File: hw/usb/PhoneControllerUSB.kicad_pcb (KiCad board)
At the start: 2 copper layers, 28.1 x 17 mm, 4 parts, among them J1 525590652, J2 DX07VN24WA2C1568

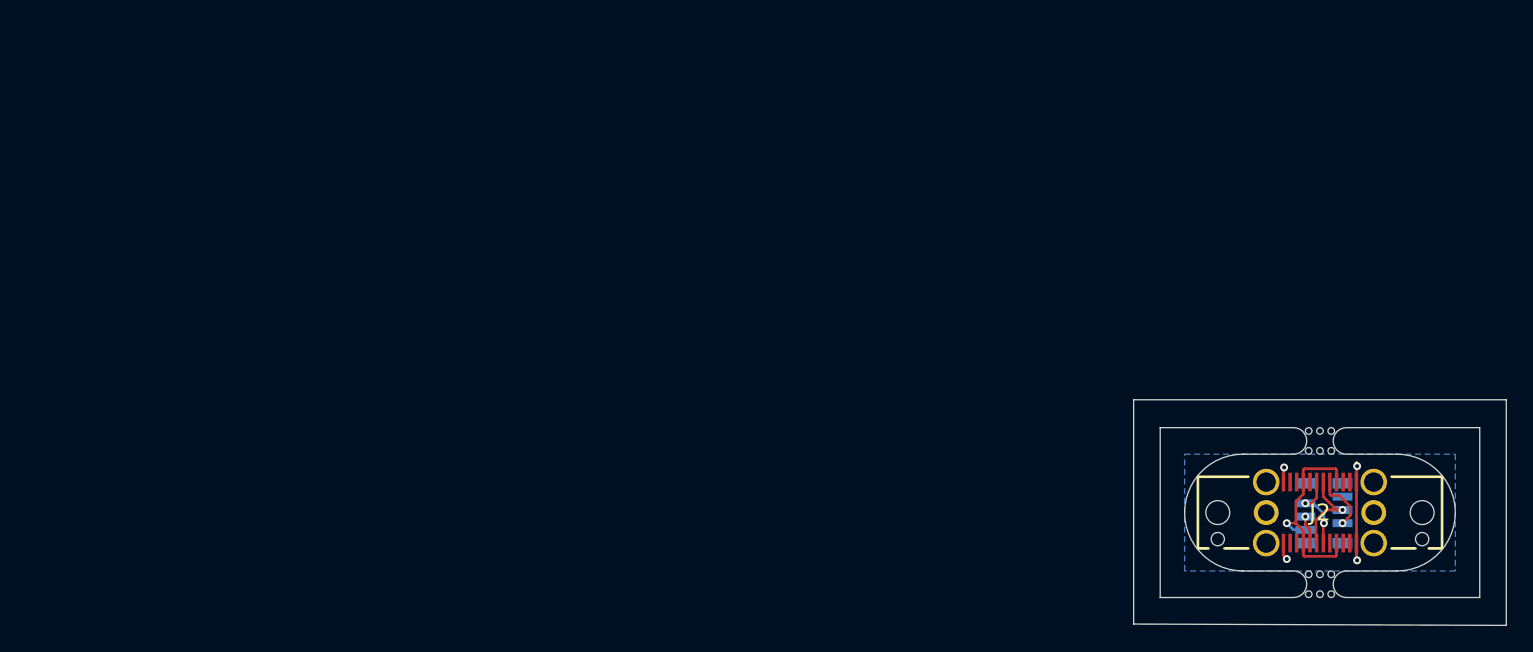
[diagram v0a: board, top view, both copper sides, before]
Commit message: chore: Updating schematics
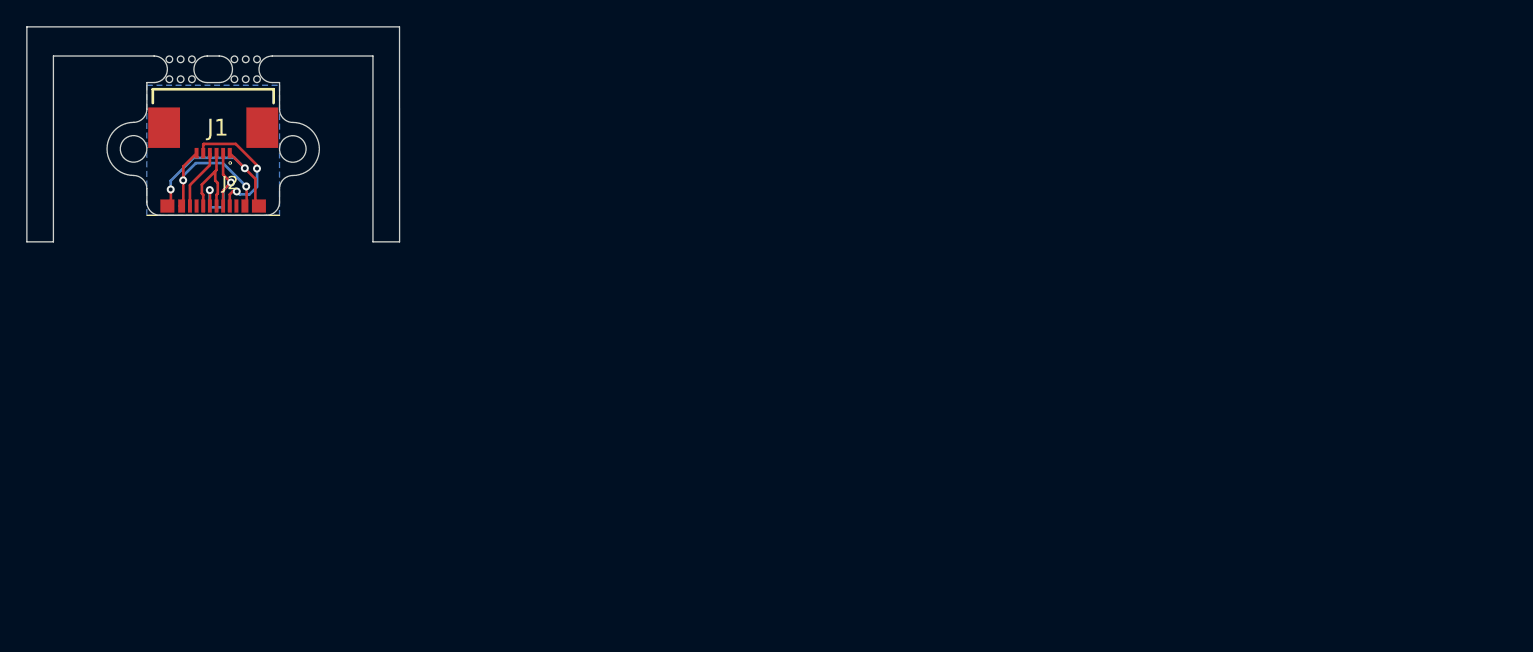
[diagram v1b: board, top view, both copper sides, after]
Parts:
- removed the REF** at (83.4, 34.0)
- removed the REF** at (83.4, 23.2)
- added REF**: MouseBite-Slot_2.0x2.0mm_outset_D0.5mm_P0.85mm_3h, Panelization:MouseBite-Slot_2.0x2.0mm_outset_D0.5mm_P0.85mm_3h, F.Cu at (2.45, -4.80)
- added REF**: MouseBite-Slot_2.0x2.0mm_outset_D0.5mm_P0.85mm_3h, Panelization:MouseBite-Slot_2.0x2.0mm_outset_D0.5mm_P0.85mm_3h, F.Cu at (-2.45, -4.80)
- J1: footprint 52559-0652:CON_525590652_MOL -> 52746-0671:52746-0671; moved to F.Cu
- J2: footprint DX07VN24WA2C1568:DX07VN24WA2C1568 -> Type-C-31-M-12:USBC1-AM-063
- moved J1 88.1 mm to (0.00, 0.00), turned to 180 degrees
- moved J2 86.4 mm to (0.00, 5.00)
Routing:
- net CC1: track 5.66 -> 10.5 mm, vias 1 -> 2
- net DM: track 6.17 -> 10.1 mm
- net VCC: track 16.2 -> 12.6 mm, vias 1 -> 2
- net GND: track 10.8 -> 14.4 mm, vias 4 -> 2
- net CC2: track 2.14 -> 4.60 mm, vias 1 -> 0
- net DP: track 7.90 -> 7.22 mm, vias 1 -> 0
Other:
- board size 28.1 x 17 mm -> 28.1 x 16.2 mm
